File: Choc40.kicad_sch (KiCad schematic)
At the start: 100 parts, among them SW1 SW_Push, SW10 SW_Push, SW11 SW_Push, SW12 SW_Push, SW13 SW_Push, SW14 SW_Push, SW15 SW_Push, SW16 SW_Push, SW17 SW_Push, SW18 SW_Push, SW19 SW_Push, SW2 SW_Push, SW20 SW_Push, SW21 SW_Push, SW22 SW_Push, SW23 SW_Push, SW24 SW_Push, SW25 SW_Push, SW26 SW_Push, SW27 SW_Push, SW28 SW_Push, SW29 SW_Push, SW3 SW_Push, SW30 SW_Push, SW31 SW_Push, SW32 SW_Push, SW33a1 SW_Push, SW33b1 SW_Push, SW34a1 SW_Push, SW34b1 SW_Push, SW35 SW_Push, SW36 SW_Push, SW37 SW_Push, SW38 SW_Push, SW39 SW_Push, SW4 SW_Push, SW40 SW_Push, SW5 SW_Push, SW6 SW_Push, SW7 SW_Push, SW8 SW_Push, SW9 SW_Push, SW99 SW_Push, U1 ATmega32U2-MU, Y1 Resonator_Small

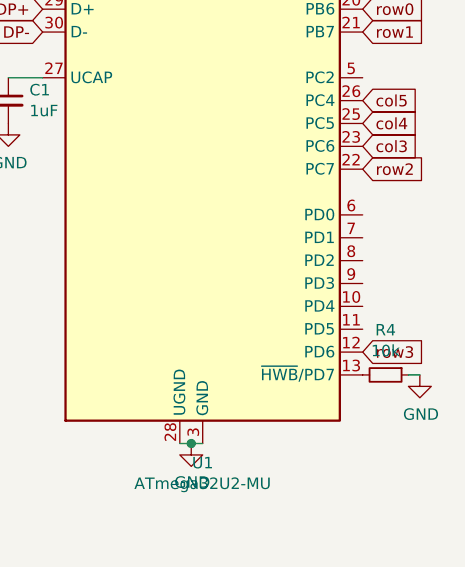
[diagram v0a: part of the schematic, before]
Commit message: Schematic finished
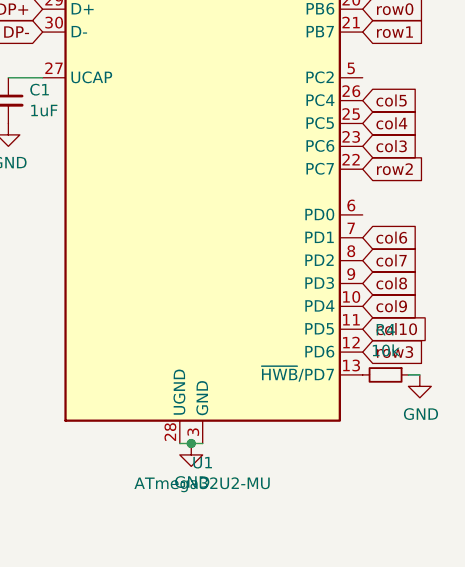
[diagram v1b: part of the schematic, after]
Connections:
- net col10: now also U1.11 (PD5)
- net col6: now also U1.7 (PD1)
- net col7: now also U1.8 (PD2)
- net col8: now also U1.9 (PD3)
- net col9: now also U1.10 (PD4)
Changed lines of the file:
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@@
+    )
+  )
+  (global_label "col6" (shape input) (at 279.4 82.55 0)
+    (effects (font (size 1.27 1.27)) (justify left))
+    (property "Intersheet References" "${INTERSHEET_REFS}" (id 0) (at 285.9255 82.4706 0)
+      (effects (font (size 1.27 1.27)) (justify left) hide)
+    )
+  )
+  (global_label "col7" (shape input) (at 279.4 85.09 0)
+    (effects (font (size 1.27 1.27)) (justify left))
+    (property "Intersheet References" "${INTERSHEET_REFS}" (id 0) (at 285.9255 85.0106 0)
+      (effects (font (size 1.27 1.27)) (justify left) hide)
+    )
+  )
+  (global_label "col8" (shape input) (at 279.4 87.63 0)
+    (effects (font (size 1.27 1.27)) (justify left))
+    (property "Intersheet References" "${INTERSHEET_REFS}" (id 0) (at 285.9255 87.5506 0)
+      (effects (font (size 1.27 1.27)) (justify left) hide)
+    )
+  )
+  (global_label "col9" (shape input) (at 279.4 90.17 0)
+    (effects (font (size 1.27 1.27)) (justify left))
+    (property "Intersheet References" "${INTERSHEET_REFS}" (id 0) (at 285.9255 90.0906 0)
+      (effects (font (size 1.27 1.27)) (justify left) hide)
+    )
+  )
+  (global_label "col10" (shape input) (at 279.4 92.71 0)
+    (effects (font (size 1.27 1.27)) (justify left))
+    (property "Intersheet References" "${INTERSHEET_REFS}" (id 0) (at 287.135 92.6306 0)
+      (effects (font (size 1.27 1.27)) (justify left) hide)
     )
   )

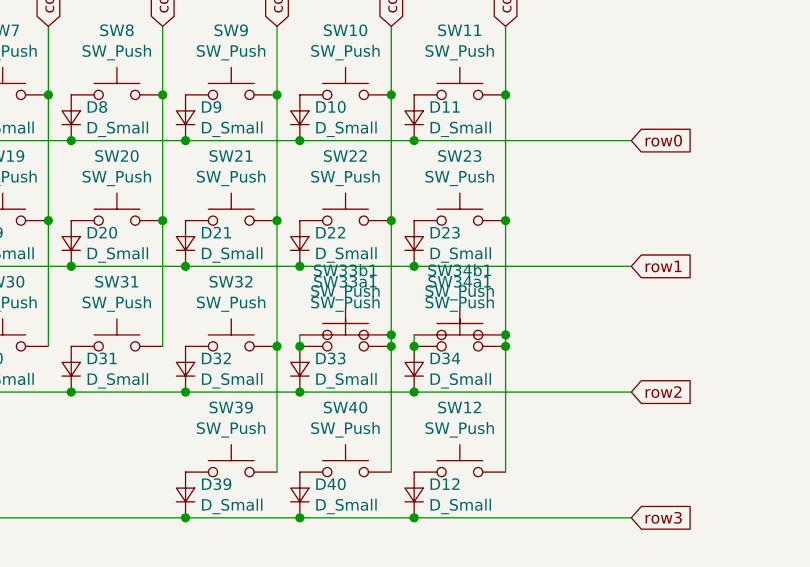
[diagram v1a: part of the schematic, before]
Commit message: Production files added
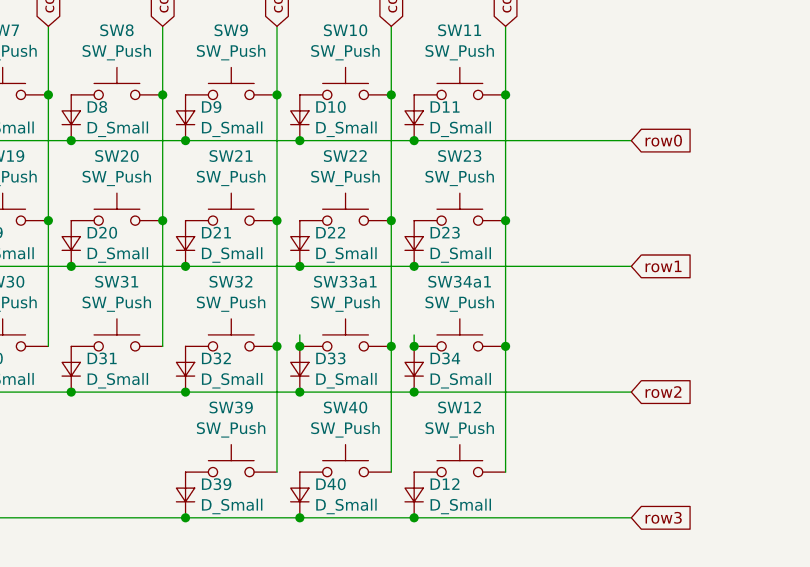
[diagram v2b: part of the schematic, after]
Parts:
- removed SW33b1: SW_Push, mbk:Choc-1.25u-solder, symbol Switch:SW_Push
- removed SW34b1: SW_Push, mbk:Choc-1u-solder, symbol Switch:SW_Push
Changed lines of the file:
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@@
   (junction (at 149.86 25.4) (diameter 1.016) (color 0 0 0 0))
   (junction (at 149.86 39.37) (diameter 1.016) (color 0 0 0 0))
-  (junction (at 149.86 52.07) (diameter 1.016) (color 0 0 0 0))
   (junction (at 149.86 53.34) (diameter 1.016) (color 0 0 0 0))
   (junction (at 152.4 30.48) (diameter 1.016) (color 0 0 0 0))
@@
   (junction (at 162.56 25.4) (diameter 1.016) (color 0 0 0 0))
   (junction (at 162.56 39.37) (diameter 1.016) (color 0 0 0 0))
-  (junction (at 162.56 52.07) (diameter 1.016) (color 0 0 0 0))
   (junction (at 162.56 53.34) (diameter 1.016) (color 0 0 0 0))
   (junction (at 191.77 154.94) (diameter 1.016) (color 0 0 0 0))
@@
     (stroke (width 0) (type solid) (color 0 0 0 0))
   )
-  (wire (pts (xy 149.86 39.37) (xy 149.86 52.07))
-    (stroke (width 0) (type solid) (color 0 0 0 0))
-  )
-  (wire (pts (xy 149.86 52.07) (xy 149.86 53.34))
+  (wire (pts (xy 149.86 39.37) (xy 149.86 53.34))
     (stroke (width 0) (type solid) (color 0 0 0 0))
   )
@@
     (stroke (width 0) (type solid) (color 0 0 0 0))
   )
-  (wire (pts (xy 162.56 39.37) (xy 162.56 52.07))
-    (stroke (width 0) (type solid) (color 0 0 0 0))
-  )
-  (wire (pts (xy 162.56 52.07) (xy 162.56 53.34))
+  (wire (pts (xy 162.56 39.37) (xy 162.56 53.34))
     (stroke (width 0) (type solid) (color 0 0 0 0))
   )
@@
     (pin "2")
   )
-  (symbol (lib_id "Switch:SW_Push") (at 144.78 52.07 0) (unit 1)
-    (in_bom yes) (on_board yes)
-    (property "Reference" "SW33b1" (id 0) (at 144.78 44.9388 0))
-    (property "Value" "SW_Push" (id 1) (at 144.78 47.2375 0))
-    (property "Footprint" "mbk:Choc-1.25u-solder" (id 2) (at 144.78 46.99 0)
-      (effects (font (size 1.27 1.27)) hide)
-    )
-    (property "Datasheet" "~" (id 3) (at 144.78 46.99 0)
-      (effects (font (size 1.27 1.27)) hide)
-    )
-    (pin "1")
-    (pin "2")
-  )
   (symbol (lib_id "Switch:SW_Push") (at 144.78 53.34 0) (unit 1)
     (in_bom yes) (on_board yes)
@@
     )
     (property "Datasheet" "~" (id 3) (at 157.48 34.29 0)
-      (effects (font (size 1.27 1.27)) hide)
-    )
-    (pin "1")
-    (pin "2")
-  )
-  (symbol (lib_id "Switch:SW_Push") (at 157.48 52.07 0) (unit 1)
-    (in_bom yes) (on_board yes)
-    (property "Reference" "SW34b1" (id 0) (at 157.48 44.9388 0))
-    (property "Value" "SW_Push" (id 1) (at 157.48 47.2375 0))
-    (property "Footprint" "mbk:Choc-1u-solder" (id 2) (at 157.48 46.99 0)
-      (effects (font (size 1.27 1.27)) hide)
-    )
-    (property "Datasheet" "~" (id 3) (at 157.48 46.99 0)
       (effects (font (size 1.27 1.27)) hide)
     )
@@
       (reference "SW33a1") (unit 1) (value "SW_Push") (footprint "mbk:Choc-1u-solder")
     )
-    (path "/80c878c1-ee97-4cff-8eb3-f2fe2237af2d"
-      (reference "SW33b1") (unit 1) (value "SW_Push") (footprint "mbk:Choc-1.25u-solder")
-    )
     (path "/09c4c897-265d-44b9-ab48-8d036398bca5"
       (reference "SW34a1") (unit 1) (value "SW_Push") (footprint "mbk:Choc-1.25u-solder")
     )
-    (path "/ce391e13-d2cb-4977-98c8-40934a09bb87"
-      (reference "SW34b1") (unit 1) (value "SW_Push") (footprint "mbk:Choc-1u-solder")
-    )
     (path "/506161a0-a779-4818-a3af-c15360bc2bfb"
